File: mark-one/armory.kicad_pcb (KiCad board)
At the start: 8 copper layers, 65.6 x 19.6 mm, 184 parts, among them J1 MICRO_SD_HINGE, J2 USB_A_PLUG, P1 TST, P10 TST, P11 TST, P12 TST, P13 TST, P2 TST, P3 TST, P4 CONN_01X07, P5 TST, P6 TST, P8 TST, P9 TST, U2 MX53, U3 NCP1529, U4 MT41K256M16HA, U5 TPD2E001DRLR, X1 32.768kHz, X2 24MHz

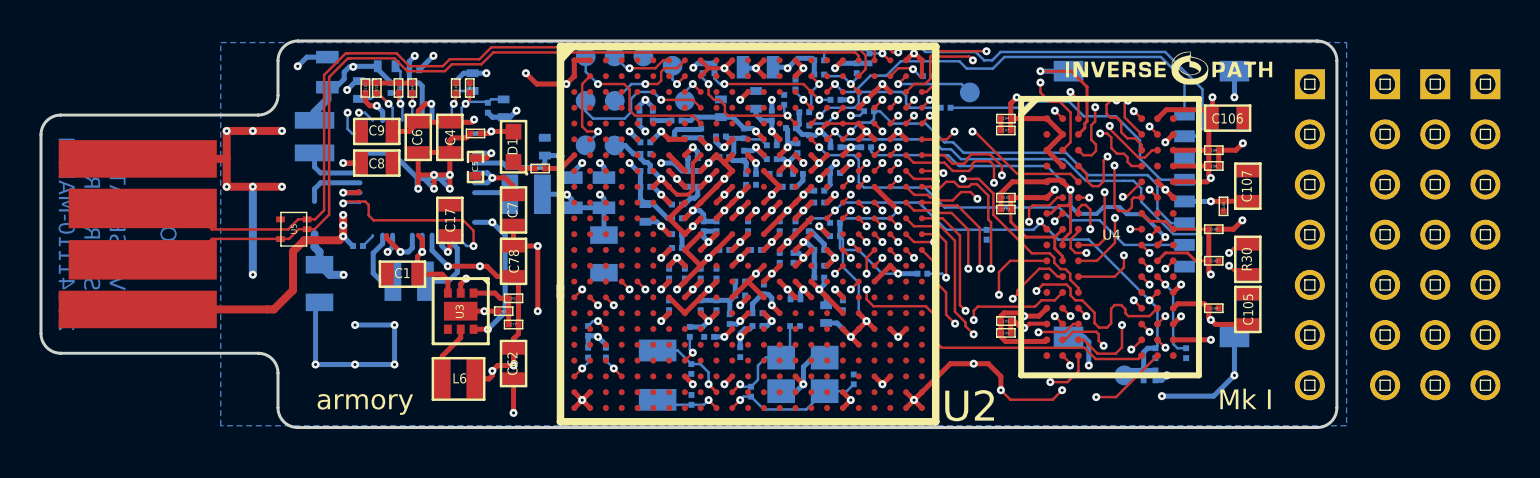
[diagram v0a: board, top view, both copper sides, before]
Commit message: modified zones
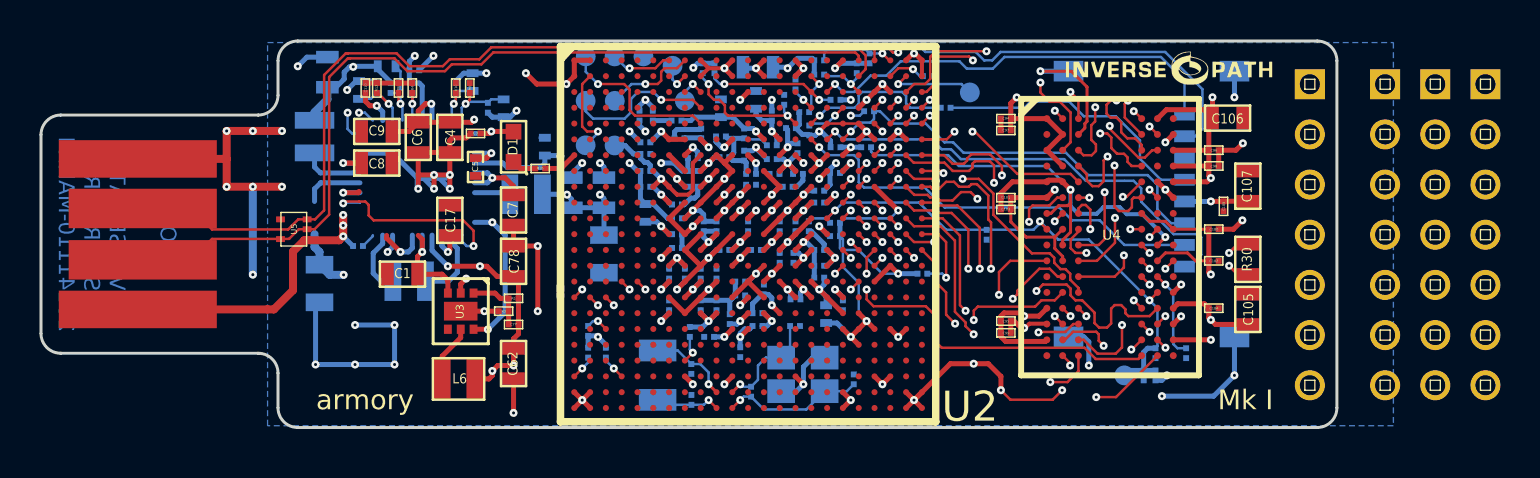
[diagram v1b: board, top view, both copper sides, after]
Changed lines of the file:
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@@
   (layers
     (0 TOP signal)
-    (1 GND_1 power hide)
+    (1 GND_1 power)
     (2 SIGNAL_1 signal)
-    (3 GND_POWER_1 power hide)
-    (4 GND_POWER_2 power hide)
-    (5 SIGNAL_2 signal hide)
-    (6 GND_2 power hide)
-    (31 BOTTOM signal hide)
+    (3 GND_POWER_1 power)
+    (4 GND_POWER_2 power)
+    (5 SIGNAL_2 signal)
+    (6 GND_2 power)
+    (31 BOTTOM signal)
     (32 B.Adhes user)
     (33 F.Adhes user)
@@
     (polygon
       (pts
-        (xy 170.2 105.1) (xy 113.2 105.1) (xy 113.2 85.7) (xy 170.2 85.7)
+        (xy 172.57 105.1) (xy 115.57 105.1) (xy 115.57 85.7) (xy 172.57 85.7)
       )
     )
@@
     (polygon
       (pts
-        (xy 170.2 105.1) (xy 104 105.1) (xy 104 85.7) (xy 170.2 85.7)
+        (xy 167.8 104.765198) (xy 101.6 104.765198) (xy 101.6 85.365198) (xy 167.8 85.365198)
       )
     )
@@
     (polygon
       (pts
-        (xy 169.4 91.4) (xy 166.15 91.4) (xy 166.15 87.75) (xy 144.8 87.75) (xy 144.8 86.4)
-        (xy 138.425 86.4) (xy 138.425 87.4) (xy 136.8 87.4) (xy 136.8 86.4) (xy 125.3 86.4)
-        (xy 125.3 88.225) (xy 127.2 88.225) (xy 127.2 90.55) (xy 126.25 90.55) (xy 126.25 92)
-        (xy 127.2 92) (xy 127.2 94.1) (xy 124.2 94.1) (xy 124.2 96.6) (xy 123.175 96.6)
-        (xy 123.175 95.575) (xy 119.1 95.575) (xy 119.1 95.075) (xy 119.1 91.4) (xy 123 91.4)
-        (xy 123 85.8) (xy 169.4 85.8)
+        (xy 169.358802 98.9) (xy 166.108802 98.9) (xy 166.108802 95.25) (xy 144.758802 95.25) (xy 144.758802 93.9)
+        (xy 138.383802 93.9) (xy 138.383802 94.9) (xy 136.758802 94.9) (xy 136.758802 93.9) (xy 125.258802 93.9)
+        (xy 125.258802 95.725) (xy 127.158802 95.725) (xy 127.158802 98.05) (xy 126.208802 98.05) (xy 126.208802 99.5)
+        (xy 127.158802 99.5) (xy 127.158802 101.6) (xy 124.158802 101.6) (xy 124.158802 104.1) (xy 123.133802 104.1)
+        (xy 123.133802 103.075) (xy 119.058802 103.075) (xy 119.058802 102.575) (xy 119.058802 98.9) (xy 122.958802 98.9)
+        (xy 122.958802 93.3) (xy 169.358802 93.3)
       )
     )
@@
     (polygon
       (pts
-        (xy 164.625 92.775) (xy 161.175 92.775) (xy 161.175 94.8) (xy 162.775 94.8) (xy 162.775 103.375)
-        (xy 147.2 103.375) (xy 147.2 85.75) (xy 164.625 85.75)
+        (xy 167.64 92.775) (xy 164.19 92.775) (xy 164.19 94.8) (xy 165.79 94.8) (xy 165.79 103.375)
+        (xy 150.215 103.375) (xy 150.215 85.75) (xy 167.64 85.75)
       )
     )
